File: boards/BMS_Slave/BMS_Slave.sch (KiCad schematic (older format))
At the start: 63 parts, among them J1 Mounting_Hole_4-40, J2 Mounting_Hole_4-40, J3 Mounting_Hole_4-40, J4 Mounting_Hole_4-40, J5 MicroFit_12, J6 MicroFit_20, J7 NanoFit_2, J8 NanoFit_2, Q1 Q_NPN_BCE, T1 T_LAN_7490100111A, U1 LTC6811-1, U2 24AA01, U3 MCP6001, U4 LTC1380, U5 LTC1380, U6 MCP6001

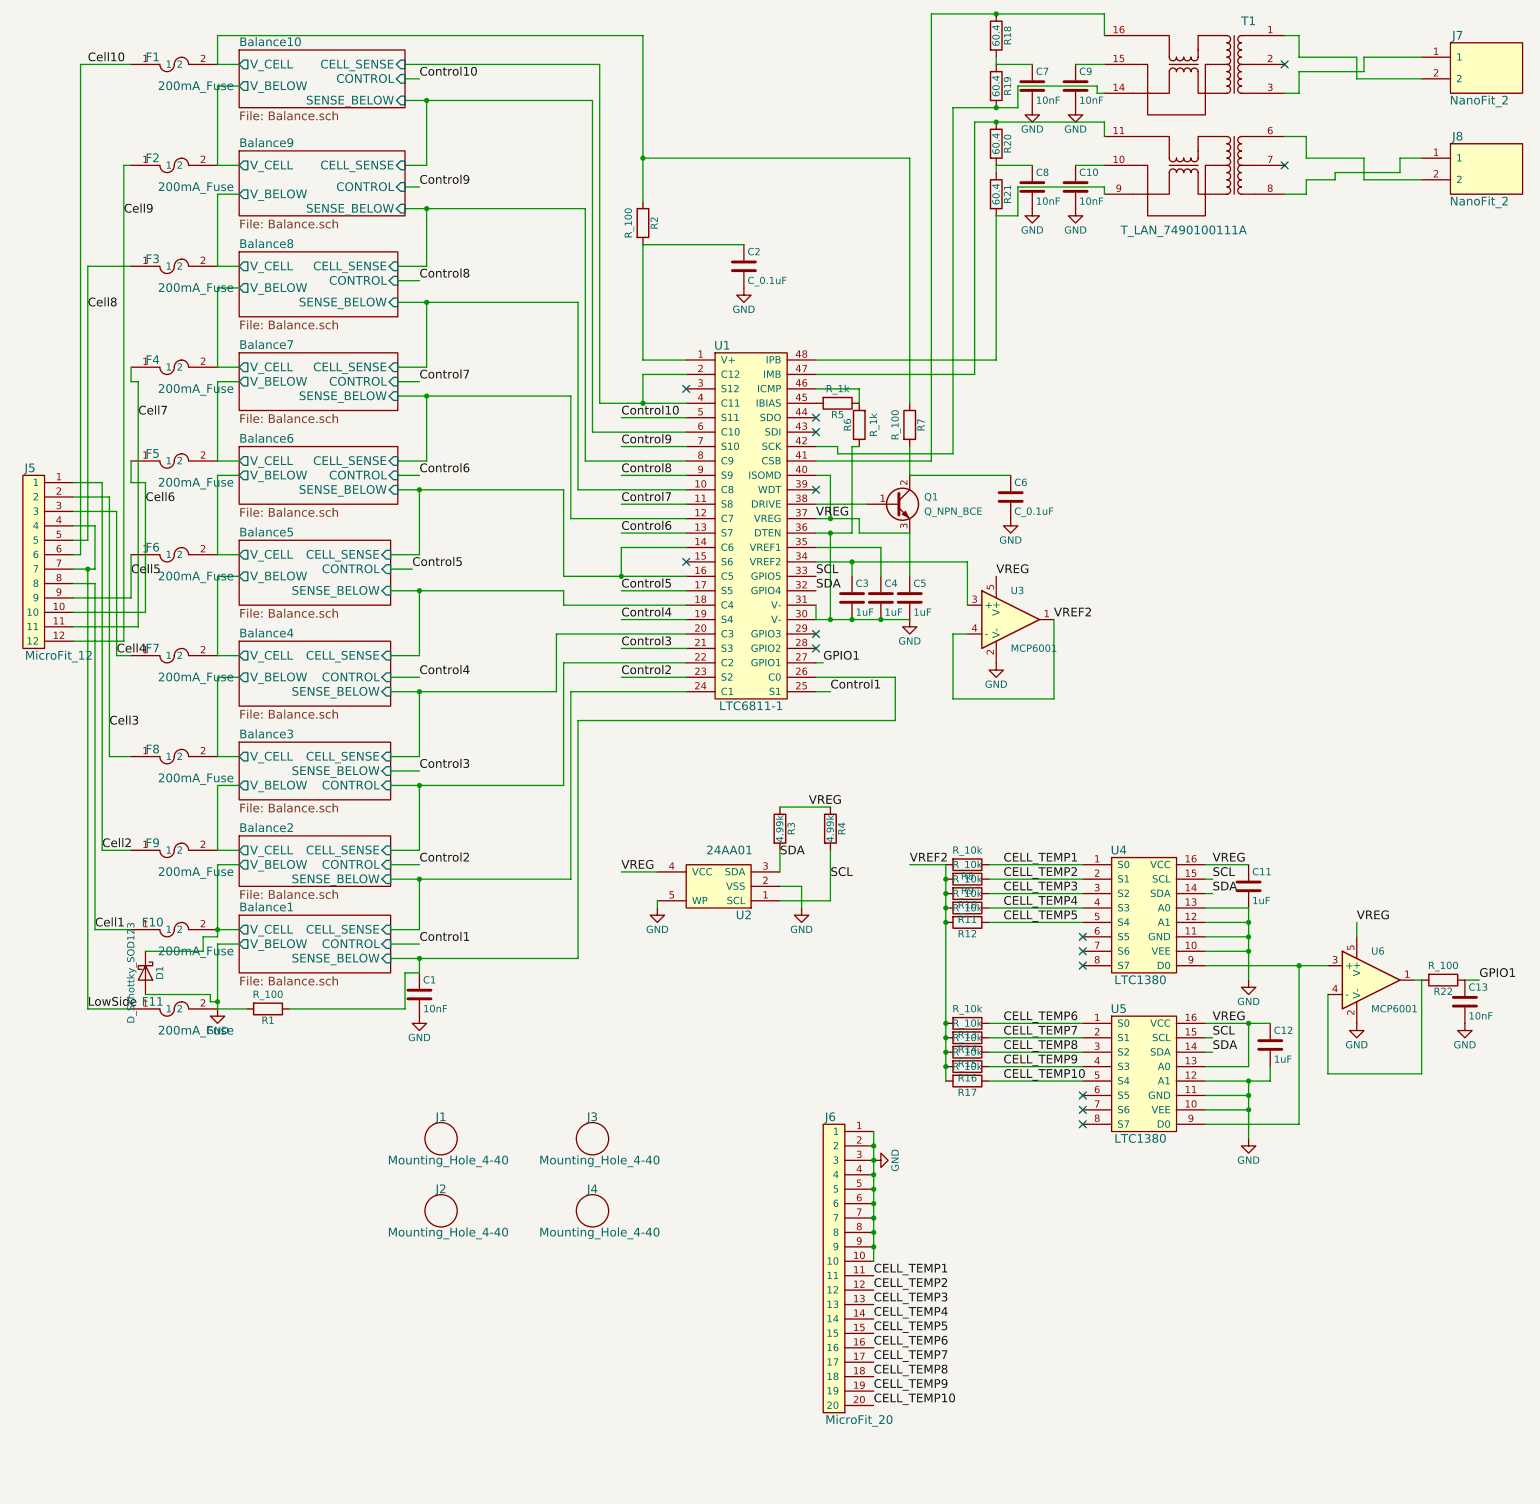
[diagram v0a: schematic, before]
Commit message: Revert "testing"
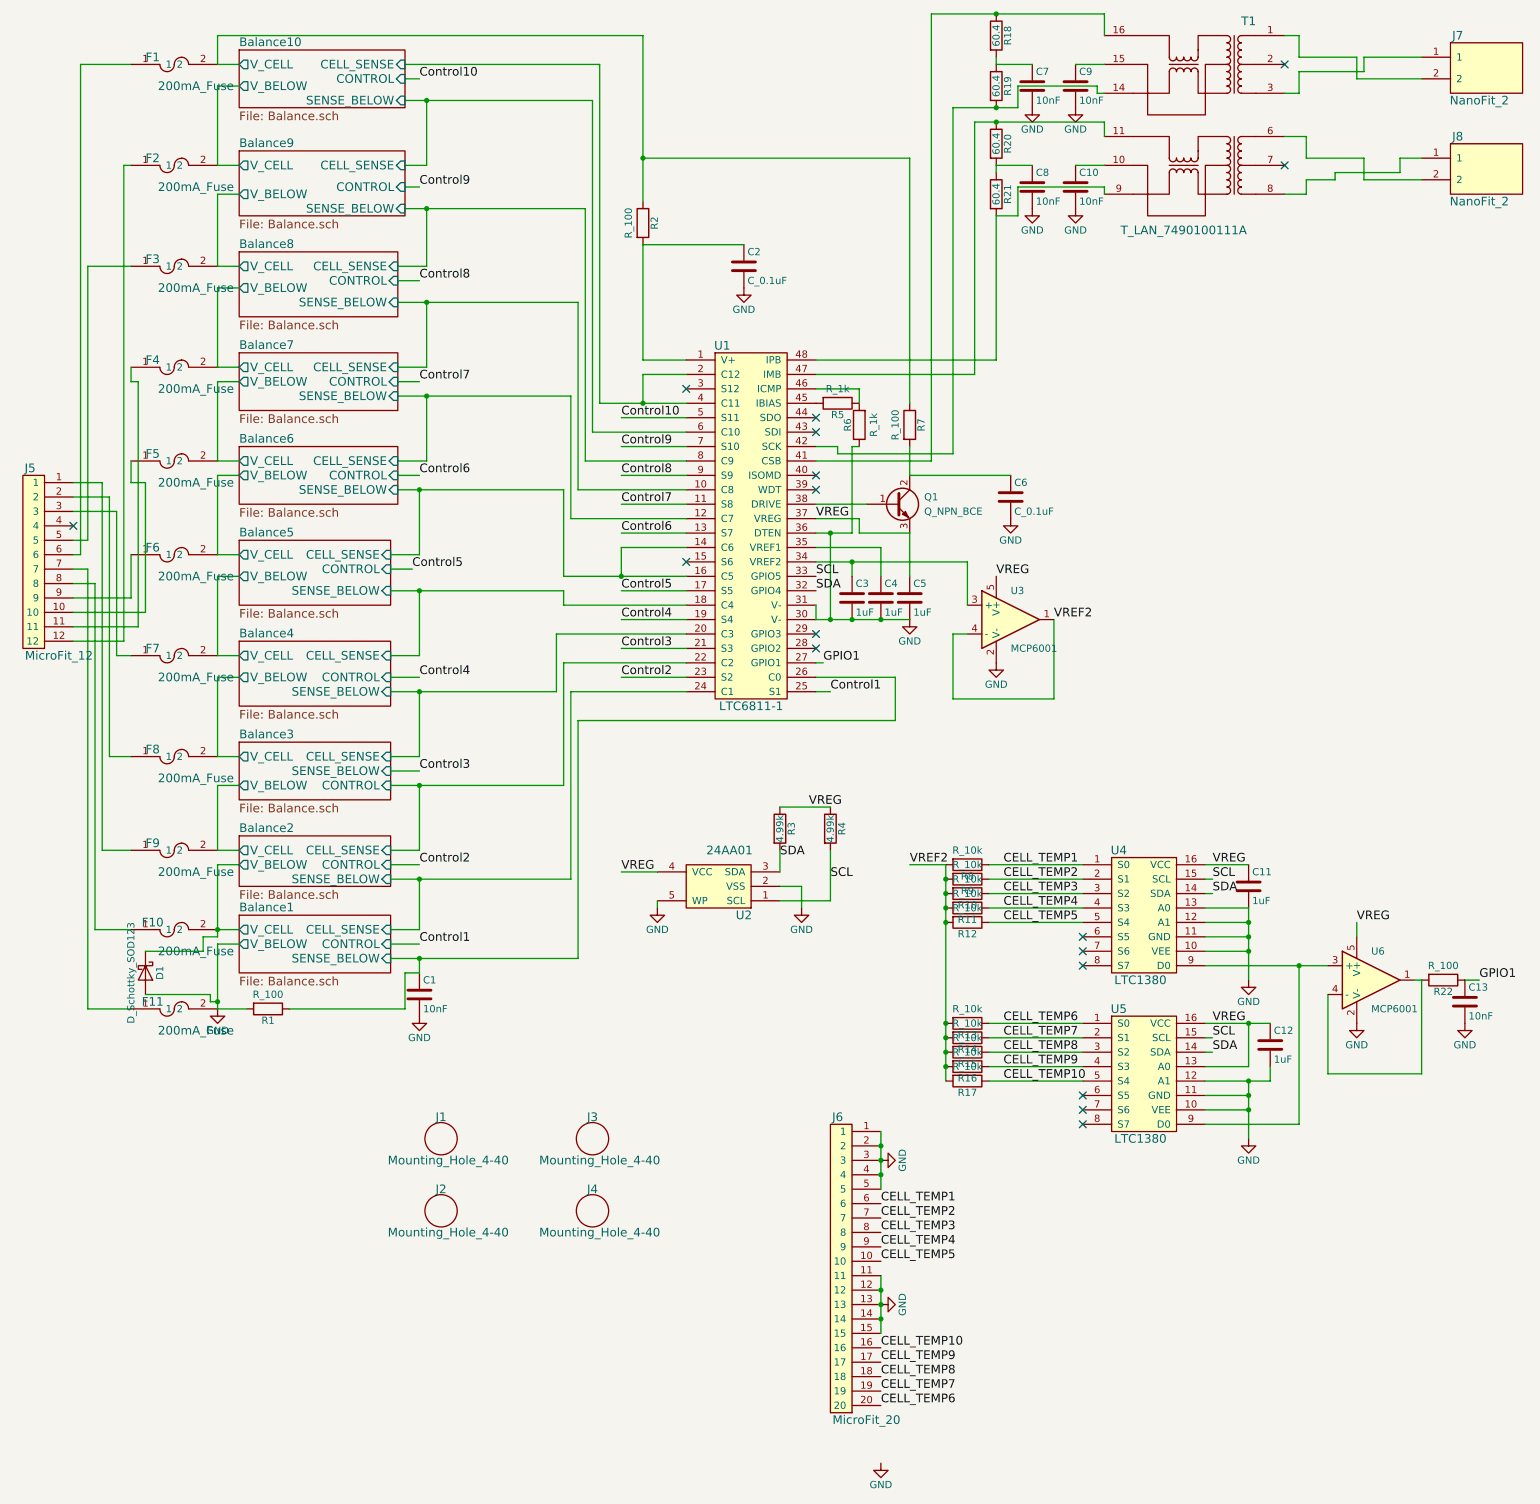
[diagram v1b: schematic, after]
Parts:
- J2, J4: footprint footprints:Mounting_Hole_Insert_4-40 -> footprints:Mounting_Hole_4-40
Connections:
- net CELL_TEMP1: now also J6.6; no longer J6.11
- net CELL_TEMP10: now also J6.16; no longer J6.20
- net CELL_TEMP2: now also J6.7; no longer J6.12
- net CELL_TEMP3: now also J6.8; no longer J6.13
- net CELL_TEMP4: now also J6.9; no longer J6.14
- net CELL_TEMP5: now also J6.10; no longer J6.15
- net CELL_TEMP6: now also J6.20; no longer J6.16
- net CELL_TEMP7: now also J6.19; no longer J6.17
- net CELL_TEMP9: now also J6.17; no longer J6.19
- net GND: now also J6.11, J6.12, J6.13, J6.14, J6.15; no longer J6.10, J6.6, J6.7, J6.8, J6.9
- net VREG: no longer U1.40 (ISOMD)
- net Cell1: no longer names the net of F10.1, J5.8
- net Cell10: no longer names the net of F1.1, J5.6
- net Cell2: no longer names the net of F9.1, J5.1
- net Cell3: no longer names the net of F8.1, J5.2
- net Cell4: no longer names the net of F7.1, J5.3
- net Cell5: no longer names the net of F6.1, J5.9
- net Cell6: no longer names the net of F5.1, J5.10
- net Cell7: no longer names the net of F4.1, J5.11
- net Cell8: no longer names the net of F3.1, J5.5
- net Cell9: no longer names the net of F2.1, J5.12
- net LowSide: no longer names the net of F11.1, J5.7
- net LowSide: no longer J5.4
- no-connect marks 15 -> 17
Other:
- moved on the sheet: J6
